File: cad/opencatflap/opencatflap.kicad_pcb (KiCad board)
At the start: 2 copper layers, 110 x 50 mm, 61 parts, among them J1 Screw_Terminal_01x02, J2 Screw_Terminal_01x04, J3 Screw_Terminal_01x01, P1 PIR Outside, P10 RFID OutSide, P11 Servo Inside, P12 Servo Outside, P2 Flap IR Inside, P4 Flap IR Outside, P9 RFID Inside, Q1 BSS138, Q2 BSS138, Q3 BSS138, Q4 BSS138, Q5 BC546B, Q6 BC546B, U1 TPS22810DRV, U2 TPS22810DRV, U3 LM1117DT-3.3, U4 LM324, U5 TCRT5000L, U6 LMR54410DBVR, U7 AMN33111

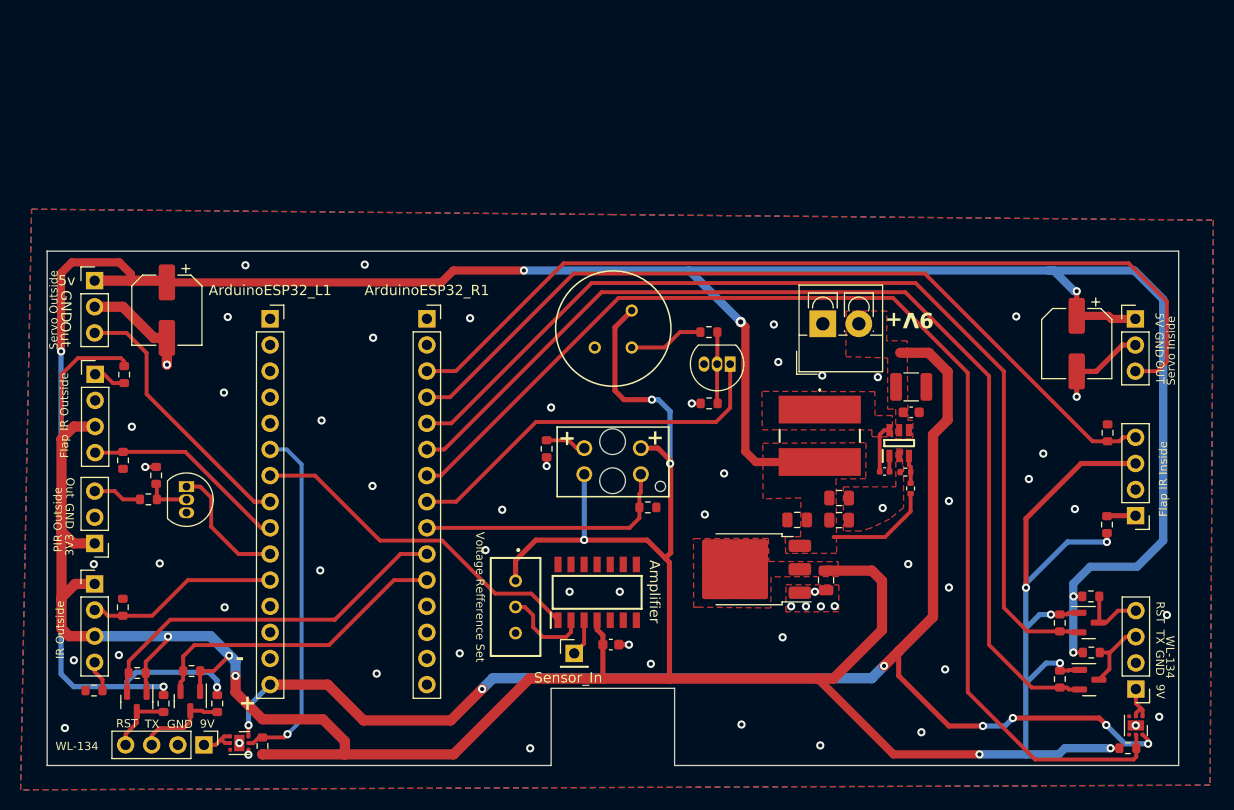
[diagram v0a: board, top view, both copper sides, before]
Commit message: update
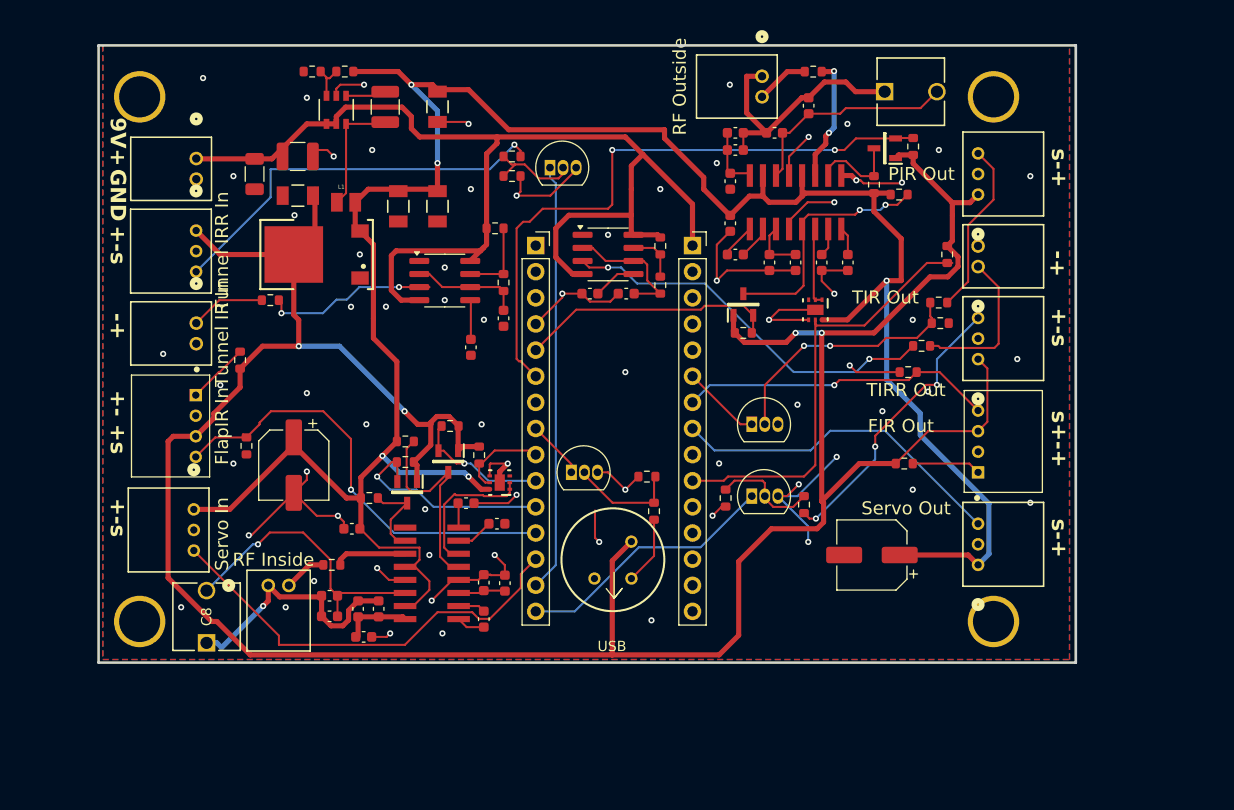
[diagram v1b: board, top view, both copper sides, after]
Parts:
- removed ArduinoESP32_L1: VIN-D13, Connector_PinSocket_2.54mm:PinSocket_1x15_P2.54mm_Vertical
- removed ArduinoESP32_R1: Pin TX1-D12, Connector_PinSocket_2.54mm:PinSocket_1x15_P2.54mm_Vertical
- removed J1: Screw_Terminal_01x02, TerminalBlock_4Ucon:TerminalBlock_4Ucon_1x02_P3.50mm_Vertical
- removed J2: Screw_Terminal_01x04, Connector_PinHeader_2.54mm:PinHeader_1x04_P2.54mm_Vertical
- removed J3: Screw_Terminal_01x01, Connector_PinHeader_2.54mm:PinHeader_1x01_P2.54mm_Vertical
- removed Q5, Q6: BC546B, Package_TO_SOT_THT:TO-92_Inline
- removed RV1: 10k, Alexander Project1:3296W-1
- added C11: 1nF, Capacitor_SMD:C_0603_1608Metric, F.Cu at (127.5, 135.5)
- added C12: 1nF, Capacitor_SMD:C_0603_1608Metric, F.Cu at (127.5, 133.5)
- added C13: 22pF, Capacitor_SMD:C_0603_1608Metric, F.Cu at (132.2, 134.8)
- added C14: 22pF, Capacitor_SMD:C_0603_1608Metric, F.Cu at (130.2, 134.8)
- added C15: 1.5nF, Capacitor_SMD:C_0603_1608Metric, F.Cu at (130.8, 137.5)
- added C16: 100nF, Capacitor_SMD:C_0603_1608Metric, F.Cu at (129.6, 127.0)
- added C17: 100nF, Capacitor_SMD:C_0603_1608Metric, F.Cu at (142.4, 135.8)
- added C18: 100nF, Capacitor_SMD:C_0603_1608Metric, F.Cu at (142.4, 132.2)
- added C19: 100nF, Capacitor_SMD:C_0603_1608Metric, F.Cu at (144.5, 132.3)
- added C20: 10nF, Capacitor_SMD:C_0603_1608Metric, F.Cu at (140.7, 124.5)
- added C21: 10nF, Capacitor_SMD:C_0603_1608Metric, F.Cu at (143.7, 126.5)
- added C22: 10nF, Capacitor_SMD:C_0603_1608Metric, F.Cu at (175.3, 101.1)
- added C23: 10nF, Capacitor_SMD:C_0603_1608Metric, F.Cu at (177.8, 101.1)
- added C24: 100nF, Capacitor_SMD:C_0603_1608Metric, F.Cu at (172.8, 101.1)
- added C25: 100nF, Capacitor_SMD:C_0603_1608Metric, F.Cu at (170.2, 101.1)
- added C26: 100nF, Capacitor_SMD:C_0603_1608Metric, F.Cu at (166.9, 100.3)
- added C27: 100nF, Capacitor_SMD:C_0603_1608Metric, F.Cu at (166.4, 97.3)
- added C28: 1.5nF, Capacitor_SMD:C_0603_1608Metric, F.Cu at (166.4, 93.2)
- added C29: 22pF, Capacitor_SMD:C_0603_1608Metric, F.Cu at (166.9, 90.2)
- added C30: 22pF, Capacitor_SMD:C_0603_1608Metric, F.Cu at (166.9, 88.5)
- added C31: 1nF, Capacitor_SMD:C_0603_1608Metric, F.Cu at (174.0, 85.9)
- added C32: 1nF, Capacitor_SMD:C_0603_1608Metric, F.Cu at (170.7, 88.5)
- added C33: 12pF - 60 pF, OpenCatFlap:VCAP_GKGXXX15_SGM, F.Cu at (181.4, 84.5)
- added C36: 10nF, Capacitor_SMD:C_0603_1608Metric, F.Cu at (152.8, 104.1)
- added C37: 1nF, Capacitor_SMD:C_0603_1608Metric, F.Cu at (156.3, 104.1)
- added C39: 10nF, Capacitor_SMD:C_0603_1608Metric, F.Cu at (141.2, 109.3)
- added C40: 1nF, Capacitor_SMD:C_0603_1608Metric, F.Cu at (144.4, 106.5)
- added P3: S4B-PH-K-S_LF__SN_, OpenCatFlap:CONN_S4B-PH-K-S_JST, F.Cu at (190.5, 118.5)
- added P5: S3B-PH-K-S LFSN, OpenCatFlap:CONN_S3B-PH-K-S_JST, F.Cu at (190.5, 130.5)
- added P6: S3B-PH-K-S LFSN, OpenCatFlap:CONN_S3B-PH-K-S_JST, F.Cu at (190.5, 94.5)
- added P7: S2B-PH-K-SLFSN, OpenCatFlap:CONN_S2B-PH-K-S_JST, F.Cu at (121.5, 132.5)
- added P8: S2B-PH-K-SLFSN, OpenCatFlap:CONN_S2B-PH-K-S_JST, F.Cu at (169.5, 83.0)
- added Pad_gge19202: Bohrloch, OpenCatFlap:Bohrloch, F.Cu at (109.0, 85.0)
- added Pad_gge19226: Bohrloch, OpenCatFlap:Bohrloch, F.Cu at (109.0, 136.0)
- added Pad_gge19274: Bohrloch, OpenCatFlap:Bohrloch, F.Cu at (192.0, 136.0)
- added Pad_gge19274: Bohrloch, OpenCatFlap:Bohrloch, F.Cu at (192.0, 85.0)
- added R17: 33kΩ, Resistor_SMD:R_0603_1608Metric, F.Cu at (186.8, 107.0)
- added R19: 33kΩ, Resistor_SMD:R_0603_1608Metric, F.Cu at (159.0, 125.3)
- added R27: 11.2k, Resistor_SMD:R_0603_1608Metric, F.Cu at (159.6, 103.3)
- added R28: 82, Resistor_SMD:R_0603_1608Metric, F.Cu at (185.0, 109.2)
- added R29: 4.7k, Resistor_SMD:R_0603_1608Metric, F.Cu at (143.5, 97.8)
- added R30: 16.5k, Resistor_SMD:R_0603_1608Metric, F.Cu at (144.4, 103.0)
- added R31: 82, Resistor_SMD:R_0603_1608Metric, F.Cu at (121.7, 104.8)
- added R32: 10k, Resistor_SMD:R_0603_1608Metric, F.Cu at (173.6, 124.6)
- added U10: SENSOR MOTION SPOT 5V BLK LENS, OpenCatFlap:AMN33111, B.Cu at (156.8, 128.2)
- added U11: EM4095, OpenCatFlap:EM4095, F.Cu at (137.4, 131.3)
- added U12: EM4095, OpenCatFlap:EM4095, F.Cu at (172.8, 95.2)
- added U13: NE555D, Package_SO:SOIC-8_3.9x4.9mm_P1.27mm, F.Cu at (138.7, 102.9)
- added U14: BC546BBK, Package_TO_SOT_THT:TO-92L_Inline, F.Cu at (168.5, 123.8)
- added U8: BC546BBK, Package_TO_SOT_THT:TO-92L_Inline, F.Cu at (168.5, 116.8)
- added U9: BC546BBK, Package_TO_SOT_THT:TO-92L_Inline, F.Cu at (151.0, 121.5)
- C1, C2, C5: value 10u -> 10uF; footprint Capacitor_SMD:C_0805_2012Metric -> OpenCatFlap:CAP_CL31A_SAM
- C10: value 100n -> 100uF; footprint Capacitor_SMD:C_0603_1608Metric -> Capacitor_SMD:CP_Elec_6.3x7.7
- C3: value 100n -> 100nF; footprint Capacitor_SMD:C_0402_1005Metric -> Capacitor_SMD:C_1210_3225Metric
- C4: value 4.7u -> 10uF; footprint Capacitor_SMD:C_1210_3225Metric -> OpenCatFlap:CAP_CL31A_SAM
- C6: value 100n -> 100nF; footprint Capacitor_SMD:C_0603_1608Metric -> Capacitor_SMD:C_1210_3225Metric
- C7: value 10u -> 4.7uF; footprint Capacitor_SMD:C_0805_2012Metric -> Capacitor_SMD:C_1206_3216Metric
- C8: value 100u -> 12pF - 60 pF; footprint Capacitor_SMD:CP_Elec_6.3x7.7 -> OpenCatFlap:VCAP_GKGXXX15_SGM
- C9: value 100u -> 100uF
- L1: value 12u -> 12uH; footprint Alexander Project1:SDR0805120ML -> OpenCatFlap:LBM2016TI20J
- P1: value PIR Outside -> S2B-PH-K-SLFSN; footprint Connector_PinHeader_2.54mm:PinHeader_1x03_P2.54mm_Vertical -> OpenCatFlap:CONN_S2B-PH-K-S_JST
- P10: value RFID OutSide -> IL-G-2P-S3T2-SA; footprint Connector_PinHeader_2.54mm:PinHeader_1x04_P2.54mm_Vertical -> OpenCatFlap:CONN_S2B-PH-K-S_JST
- P11: value Servo Inside -> S2B-PH-K-SLFSN; footprint Connector_PinHeader_2.54mm:PinHeader_1x03_P2.54mm_Vertical -> OpenCatFlap:CONN_S2B-PH-K-S_JST
- P12: value Servo Outside -> S3B-PH-K-S LFSN; footprint Connector_PinHeader_2.54mm:PinHeader_1x03_P2.54mm_Vertical -> OpenCatFlap:CONN_S3B-PH-K-S_JST
- P2: value Flap IR Inside -> S4B-PH-K-S_LF__SN_; footprint Connector_PinHeader_2.54mm:PinHeader_1x04_P2.54mm_Vertical -> OpenCatFlap:CONN_S4B-PH-K-S_JST
- P4: value Flap IR Outside -> S3B-PH-K-S LFSN; footprint Connector_PinHeader_2.54mm:PinHeader_1x04_P2.54mm_Vertical -> OpenCatFlap:CONN_S3B-PH-K-S_JST
- P9: value RFID Inside -> S3B-PH-K-S LFSN; footprint Connector_PinHeader_2.54mm:PinHeader_1x04_P2.54mm_Vertical -> OpenCatFlap:CONN_S3B-PH-K-S_JST
- Q1, Q2, Q3, Q4: value BSS138 -> BSS138L; footprint Package_TO_SOT_SMD:SOT-23 -> OpenCatFlap:BSS138L
- R1: value 200R -> 118kΩ
- R10: value 118k -> 10kΩ; footprint Resistor_SMD:R_0402_1005Metric -> Resistor_SMD:R_0603_1608Metric
- R11, R14, R15, R3, R4, R6: value 10k -> 10kΩ
- R13, R16: value 10k -> 560Ω
- R18, R20, R24, R25: value 10k -> 33kΩ
- R2: value 33k -> 22.1kΩ
- R21: value 566R -> 27Ω
- R22: value 10k -> 27Ω
- R23: value 22.1k -> 10k; footprint Resistor_SMD:R_0402_1005Metric -> Resistor_SMD:R_0603_1608Metric
- R26: value 200R -> 3.3k
- R5: value 566R -> 10kΩ
- R7, R8, R9: value 33k -> 10kΩ
- U1: value TPS22810DRV -> ARDUINO_NANO; footprint Package_SON:WSON-6-1EP_2x2mm_P0.65mm_EP1x1.6mm -> OpenCatFlap:Arduino Nano ESP32
- U2: value TPS22810DRV -> LM1117DTX-3.3/NOPB; footprint Package_SON:WSON-6-1EP_2x2mm_P0.65mm_EP1x1.6mm -> OpenCatFlap:LM1117DTX-3.3NOPB
- U3: value LM1117DT-3.3 -> LMR54410DBVR; footprint Package_TO_SOT_SMD:TO-252-3_TabPin2 -> OpenCatFlap:U_SOT-23_TEX
- U4: value LM324 -> BC546BBK; footprint Alexander Project1:SOIC127P600X175-14N -> Package_TO_SOT_THT:TO-92L_Inline
- U5: value TCRT5000L -> NE555D; footprint Alexander Project1:TCRT5000L -> Package_SO:SOIC-8_3.9x4.9mm_P1.27mm; moved to F.Cu
- U6: value LMR54410DBVR -> TPS22810DRVR; footprint Alexander Project1:LMR54410DBVR -> OpenCatFlap:DRV0006A_NV
- U7: value AMN33111 -> TPS22810DRVR; footprint Alexander Project1:AMN33111 -> OpenCatFlap:DRV0006A_NV; moved to F.Cu
- moved P9 101.6 mm to (114.5, 98.0), turned to -90 degrees
- moved U2 91.9 mm to (126.1, 100.3), turned to 180 degrees
- moved P2 91.8 mm to (114.5, 117.0), turned to -90 degrees
- moved P11 91.3 mm to (114.5, 107.0), turned to -90 degrees
- moved R4 88.6 mm to (187.5, 100.3), turned to 90 degrees
- moved P10 88.5 mm to (190.5, 101.5), turned to 90 degrees
- moved P12 86.2 mm to (190.5, 110.5), turned to 90 degrees
- moved R13 83.7 mm to (118.8, 110.6), turned to 90 degrees
- moved R14 83.4 mm to (119.4, 118.9), turned to -90 degrees
- moved R8 81.9 mm to (184.2, 89.8), turned to -90 degrees
- moved R18 80.2 mm to (186.7, 105.0), turned to 0 degrees
- moved C9 77.0 mm to (124.0, 120.8)
- moved R22 77.0 mm to (174.5, 82.5), turned to 0 degrees
- moved R16 72.2 mm to (183.3, 120.7), turned to 0 degrees
- moved R26 70.0 mm to (159.6, 99.5), turned to 90 degrees
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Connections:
- C10 pad 1: +3V3 -> +5V
- C3 pad 1: /SW -> Net-(U3-CB)
- C3 pad 2: /CB -> Net-(U3-SW)
- C4 pad 1: +9V -> +5V
- C6 pad 1: +9V -> GND
- C6 pad 2: GND -> +9V
- C7 pad 1: +5V -> GND
- C7 pad 2: GND -> +9V
- C8 pad 1: +5V -> Net-(C11-Pad1)
- C8 pad 2: GND -> Net-(C11-Pad2)
- L1 pad 1: /SW -> Net-(U3-SW)
- P1 pad 1: +3V3 -> +9V
- P10 pad 1: RFID_Outside_Vin -> Net-(P10-Pad1)
- P11 pad 1: +5V -> Net-(P11-Pad1)
- P12 pad 1: +5V -> +3V3
- P12 pad 3: Servo_Outside_PWM -> Net-(P12-Pad3)
- P2 pad 1: Net-(P2-E+) -> Net-(P2-Pad1)
- P4 pad 1: Net-(P4-E+) -> +5V
- P4 pad 3: +3V3 -> Servo_Inside_PWM
- P9 pad 1: RFID_Inside_Vin -> +3V3
- P9 pad 3: RFID_Inside_5VIN -> Net-(P9-Pad3)
- Q1 pad 2: RFID_Inside_3v3VIN -> RFID_Inside_3.3VCLK
- Q1 pad 3: RFID_Inside_5VIN -> RFID_Inside_5VCLK
- Q2 pad 2: RFID_Inside_3.3VRST -> RFID_Outside_3.3VCLK
- Q2 pad 3: RFID_Inside_5VRST -> RFID_Outside_5VCLK
- Q3 pad 2: RFID_Outside_3v3VIN -> RFID_Outside_3v3VDMOD
- Q3 pad 3: RFID_Outside_5VIN -> RFID_Outside_5VDMOD
- Q4 pad 2: RFID_Outside_3.3VRST -> RFID_Inside_3.3VDMOD
- Q4 pad 3: RFID_Outside_5VRST -> RFID_Inside_5VDMOD
- R1 pad 1: Net-(R1-Pad1) -> Net-(U3-FB)
- R1 pad 2: GND -> +5V
- R10 pad 1: +5V -> RFID_Outside_5VDMOD
- R10 pad 2: /FB -> +5V
- R11 pad 1: +3V3 -> RFID_Inside_5VDMOD
- R11 pad 2: RFID_Inside_3v3VIN -> +5V
- R12 pad 1: +5V -> RFID_Inside_3.3VDMOD
- R12 pad 2: RFID_Inside_5VIN -> +3V3
- R13 pad 2: RFID_Inside_3.3VRST -> Net-(P2-Pad1)
- R14 pad 1: +5V -> Flap_IR_Inside
- R14 pad 2: RFID_Inside_5VRST -> GND
- R15 pad 1: +3V3 -> Flap_IR_Outside
- R15 pad 2: RFID-Inside-EN -> GND
- R16 pad 2: RFID_Outside_3v3VIN -> Net-(P3-Pad1)
- R18 pad 1: +5V -> Net-(U8-B)
- R18 pad 2: RFID_Outside_5VIN -> Net-(P6-Pad3)
- R2 pad 1: /PIR_Out -> GND
- R2 pad 2: Net-(Q6-B) -> Net-(U3-FB)
- R20 pad 1: +3V3 -> Net-(U9-B)
- R20 pad 2: RFID-Outside-EN -> GND
- R21 pad 1: Net-(P4-E+) -> Net-(P7-Pad2)
- R21 pad 2: +3V3 -> Net-(R21-Pad2)
- R22 pad 1: Flap_IR_Outside -> Net-(P8-Pad2)
- R22 pad 2: GND -> Net-(R22-Pad2)
- R23 pad 1: /FB -> Net-(U4-B)
- R23 pad 2: GND -> Net-(P9-Pad3)
- R24 pad 1: Flap_IR_Inside -> Net-(U4-B)
- R25 pad 1: IR_Outside -> Net-(U14-B)
- R26 pad 1: Net-(J2-Pin_4) -> Net-(U5-DIS)
- R26 pad 2: GND -> +9V
- R3 pad 1: TCRT5000L -> RFID-Inside-EN
- R3 pad 2: GND -> +3V3
- R4 pad 1: +3V3 -> RFID-Outside-EN
- R4 pad 2: RFID_Outside_3.3VRST -> +3V3
- R5 pad 1: Net-(P2-E+) -> RFID_Inside_3.3VCLK
- R6 pad 1: +5V -> RFID_Inside_5VCLK
- R6 pad 2: RFID_Outside_5VRST -> +5V
- R7 pad 1: Net-(Q6-B) -> RFID_Outside_5VCLK
- R7 pad 2: GND -> +5V
- R8 pad 1: Net-(P1-In) -> RFID_Outside_3.3VCLK
- R8 pad 2: Net-(Q5-B) -> +3V3
- R9 pad 1: Net-(Q5-B) -> RFID_Outside_3v3VDMOD
- R9 pad 2: GND -> +3V3
- U1 pad 1: RFID_Outside_Vin -> unconnected-(U1-D1/TX-Pad1)
- U1 pad 2: RFID_Outside_Vin -> unconnected-(U1-D0/RX-Pad2)
- U1 pad 5: RFID-Outside-EN -> RFID_Outside_3v3VDMOD
- U1 pad 6: +9V -> RFID_Outside_3.3VCLK
- U1 pad 7: GND -> unconnected-(U1-D4-Pad7)
- U2 pad 1: RFID_Inside_Vin -> GND
- U2 pad 3: unconnected-(U2-CT-Pad3) -> +5V
- U2 pad 4: GND -> +3V3
- U3 pad 1: GND -> Net-(U3-CB)
- U3 pad 2: +3V3 -> GND
- U3 pad 3: +5V -> Net-(U3-FB)
- U4 pad 1: Amplifier_Out -> Tunnel_IR_IN
- U4 pad 2: Net-(U4A--) -> Net-(U4-B)
- U4 pad 3: Net-(J3-Pin_1) -> GND
- U5 pad 1: +3V3 -> GND
- U5 pad 2: TCRT5000L -> Net-(U5-THR)
- U5 pad 3: +3V3 -> Net-(U5-Q)
- U5 pad 4: Net-(R1-Pad1) -> +9V
- U6 pad 1: /CB -> RFID-Inside-SHDN
- U6 pad 2: GND -> RFID-Inside-SHDN
- U6 pad 3: /FB -> unconnected-(U6-CT-Pad3)
- U6 pad 4: +9V -> GND
- U6 pad 5: +9V -> RFID-Inside-EN
- U6 pad 6: /SW -> +5V
- U7 pad 1: +3V3 -> RFID-Outside-SHDN
- U7 pad 2: /PIR_Out -> RFID-Outside-SHDN
- U7 pad 3: GND -> unconnected-(U7-CT-Pad3)
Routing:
- net GND: track 24.4 -> 143.7 mm, vias 60 -> 69
- net RFID-Inside-EN: track 115.2 -> 8.72 mm
- net RFID_Inside_3v3VIN: track 101.1 -> 0.00 mm
- net RFID_Inside_3.3VRST: track 96.6 -> 0.00 mm
- net +3V3: track 333.2 -> 265.4 mm, vias 12 -> 4
- net RFID_Outside_3.3VCLK: track 0.00 -> 60.5 mm, vias 0 -> 2
- net Servo_Inside_PWM: track 87.1 -> 42.3 mm
- net Tunnel_IR_IN: track 0.00 -> 41.6 mm
- net +5V: track 267.5 -> 228.0 mm, vias 8 -> 5
- net Net-(P9-Pad3): track 0.00 -> 39.0 mm, vias 0 -> 1
- net Net-(U5-Q): track 0.00 -> 37.7 mm, vias 0 -> 2
- net Flap_IR_Inside: track 80.8 -> 43.2 mm, vias 0 -> 1
- net RFID_Outside_3.3VRST: track 36.4 -> 0.00 mm
- net Amplifier_Out: track 33.8 -> 0.00 mm
- net PIR_IN1: track 37.5 -> 5.69 mm
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- removed copper zone on F.Cu, net +3V3
- removed copper zone on F.Cu, net +5V
- removed copper zone on F.Cu, net +9V
- removed copper zone on F.Cu, net /SW
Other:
- board size 110 x 50 mm -> 95 x 60 mm
- board text added: "+-"
- board text added: "+- +s"
- board text added: "+-s"
- board text added: "-+"
- board text added: "s+-+"
- board text added: "s-+"
- board text removed: "+"
- board text removed: "-"
- board text removed: "3V3"
- board text removed: "5V"
- board text removed: "5v"
- board text removed: "9V"
- board text removed: "Amplifier"
- board text removed: "IR Outside"
- board text removed: "OUT"
- board text removed: "Out"
- board text removed: "PIR Outside"
- board text removed: "RST"
- board text removed: "Sensor_In"
- board text removed: "Servo Inside"
- board text removed: "Servo Outside"
- board text removed: "TX"
- board text removed: "Voltage Refference Set"
- board text removed: "WL-134"
